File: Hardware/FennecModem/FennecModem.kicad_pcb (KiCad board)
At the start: 2 copper layers, 70 x 116.7 mm, 15 parts, among them J101 USB_C_Receptacle_USB2.0, J201 Conn_Coaxial, U101 ATmega32U4-A, U201 DRA818V

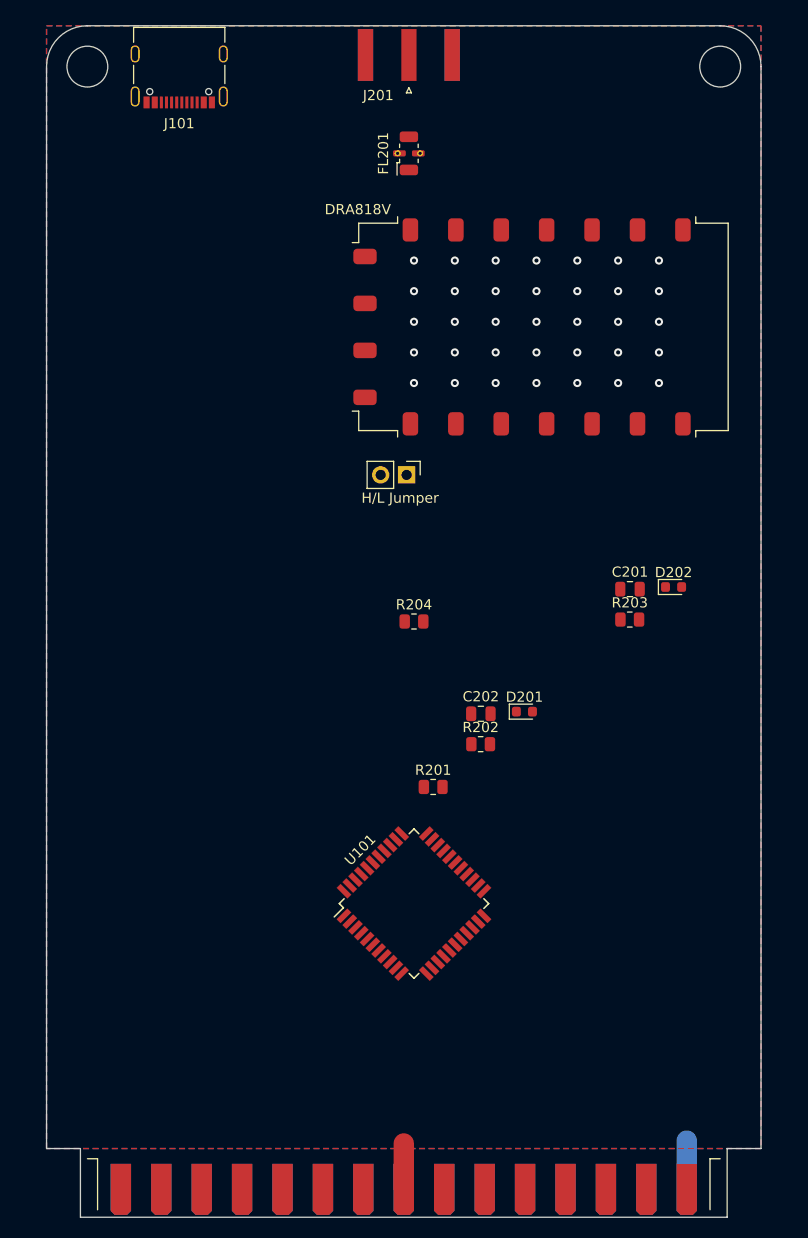
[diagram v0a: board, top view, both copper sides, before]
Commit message: Bump kenwoodfox libs
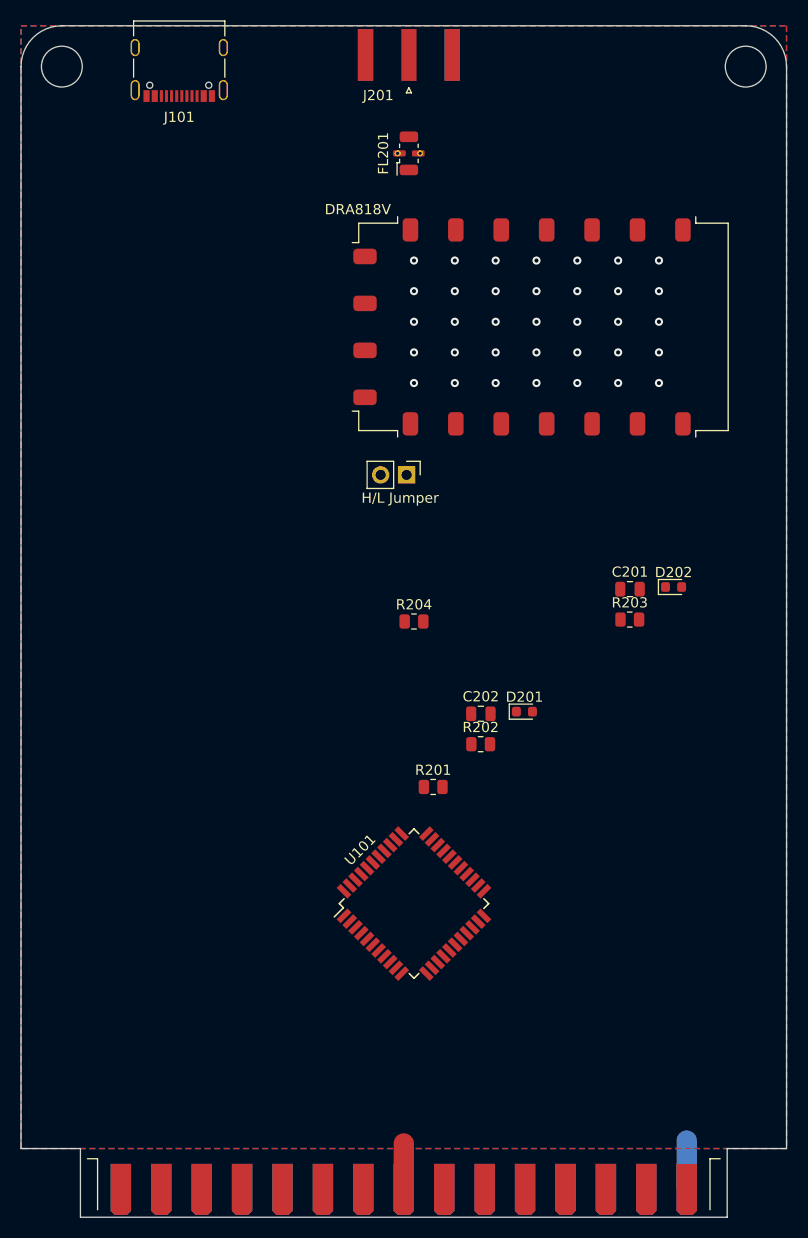
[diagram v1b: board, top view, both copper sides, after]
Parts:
- moved J101 0.62 mm to (128.0, 44.4)
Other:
- board size 70 x 116.7 mm -> 75 x 116.7 mm
